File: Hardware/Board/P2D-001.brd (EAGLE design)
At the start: 45 x 45 mm, 21 parts, among them IC1 LTC485N, K1 G5V1, T1 2SC1815

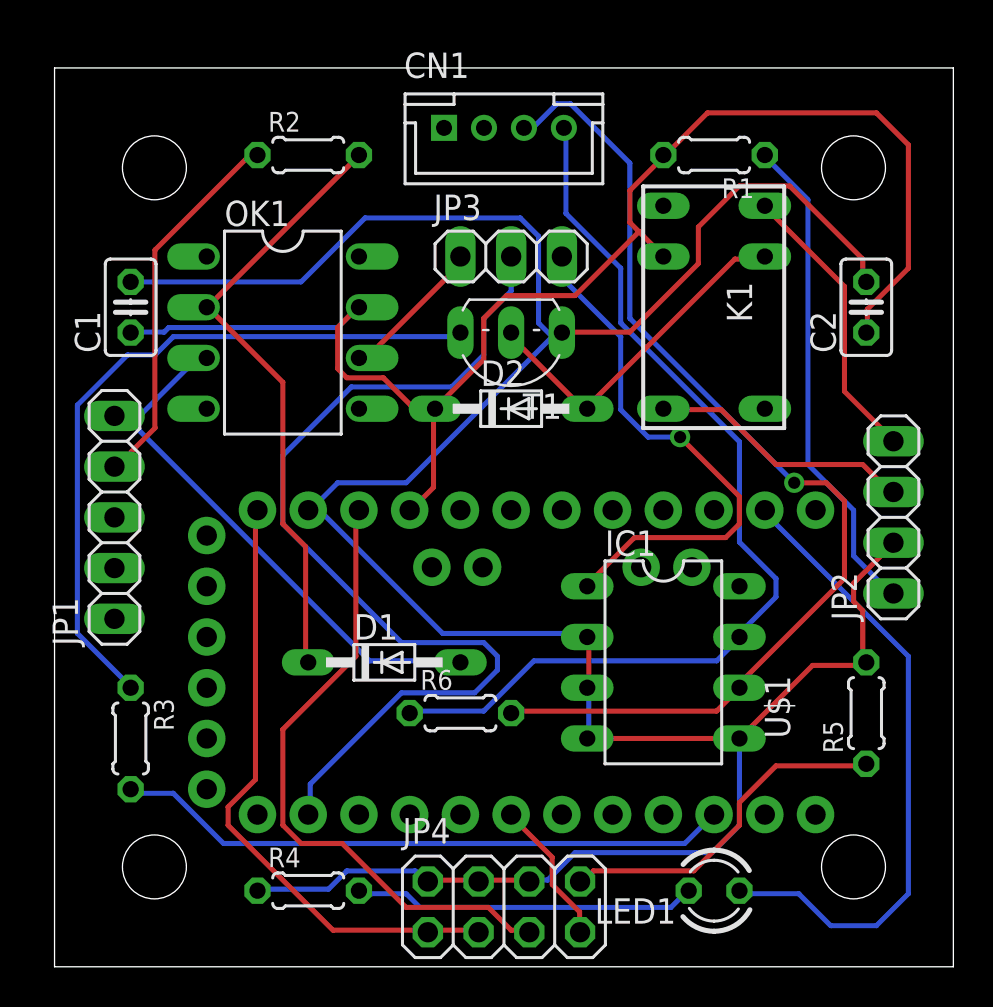
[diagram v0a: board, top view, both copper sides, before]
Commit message: Overhaul.
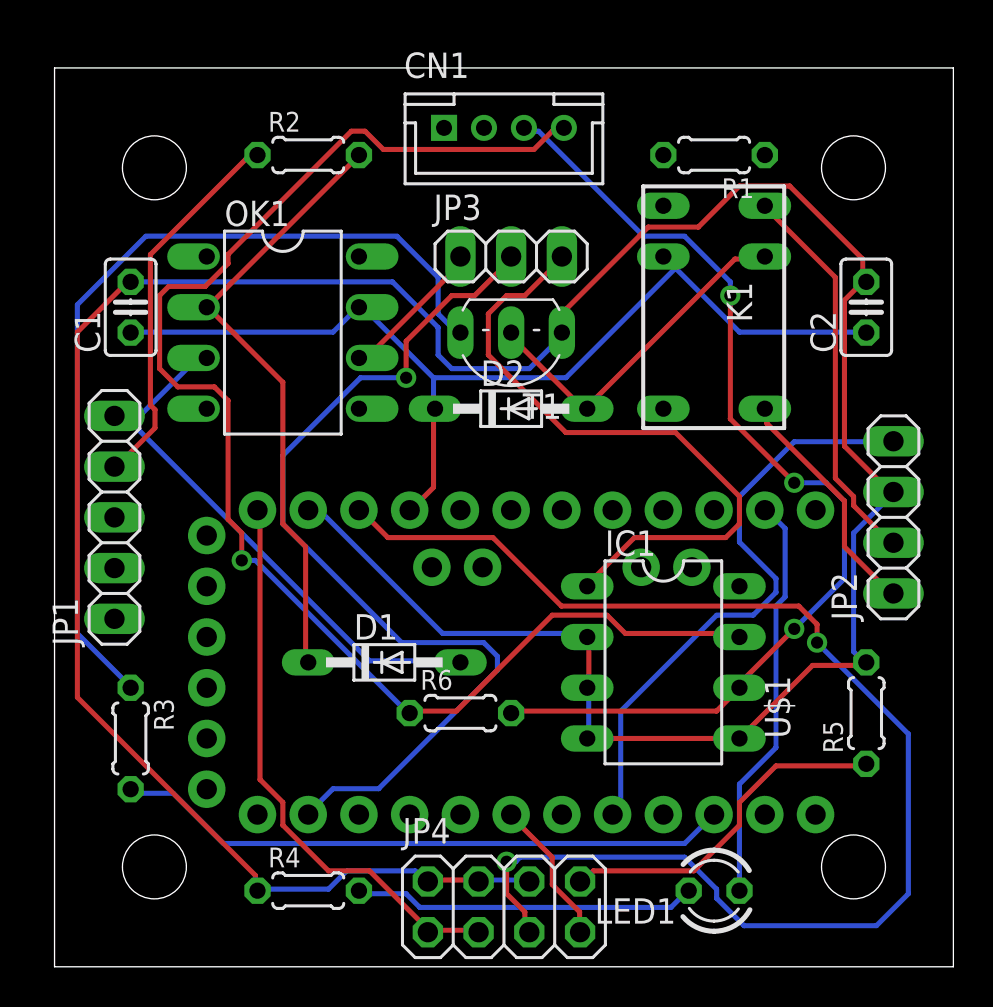
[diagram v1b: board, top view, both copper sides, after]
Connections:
- net GND: now also JP2.3; no longer JP2.2
- net N$10: now also JP2.4, U$1.8; no longer JP2.1, R1.1
- net N$18: now also JP2.1, K1.6; no longer JP2.3, K1.5
- net N$19: now also JP2.2; no longer JP2.4
- net VCC: no longer R1.2
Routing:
- net N$6: track 32.0 -> 67.3 mm, vias 0 -> 2
- net N$11: track 48.8 -> 71.5 mm, vias 0 -> 1
- net VCC: track 72.5 -> 51.4 mm
- net GND: track 141.5 -> 155.4 mm
- net N$16: track 32.3 -> 20.5 mm
- net N$13: track 35.9 -> 43.9 mm
- net N$14: track 27.0 -> 32.8 mm, vias 1 -> 0
- net N$10: track 24.7 -> 30.0 mm
- net N$19: track 14.4 -> 19.6 mm
- net N$9: track 31.3 -> 28.5 mm
- net N$20: track 48.5 -> 46.8 mm, vias 0 -> 1
- net N$2: track 52.9 -> 51.4 mm, vias 1 -> 3
- net N$18: track 13.2 -> 12.0 mm
